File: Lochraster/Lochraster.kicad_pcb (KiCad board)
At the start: 2 copper layers, 54.6 x 53.3 mm, 25 parts, among them J1 Conn_01x04_Pin, J2 Conn_01x32_Pin, J3 Conn_01x04_Pin, J4 Conn_01x07_Pin, J5 Conn_01x08_Pin, J6 Conn_01x04_Pin, J7 Conn_01x08_Pin, J8 Conn_01x04_Pin, J9 Conn_01x04_Pin

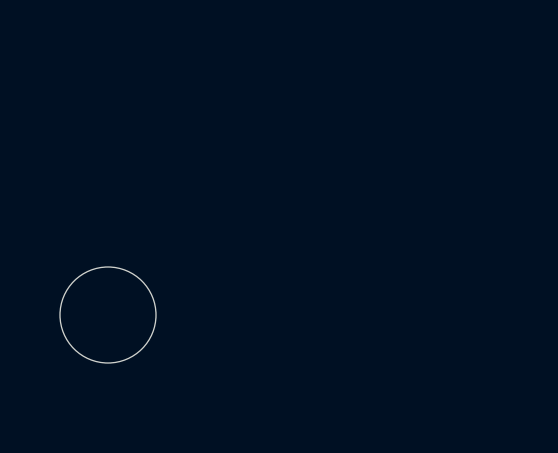
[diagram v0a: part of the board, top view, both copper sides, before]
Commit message: final version V1.0
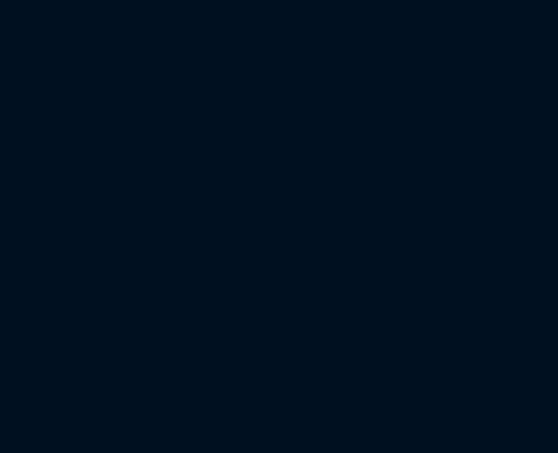
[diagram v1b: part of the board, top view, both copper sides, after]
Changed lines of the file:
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@@
     (property "ki_description" "Generic connector, single row, 01x04, script generated")
     (property "ki_keywords" "connector")
-    (attr through_hole)
+    (attr through_hole exclude_from_pos_files)
     (fp_text reference "J6" (at 0 -2.77 90) (layer "F.SilkS") hide
         (effects (font (size 1 1) (thickness 0.15)))
@@
     (property "ki_description" "Generic connector, single row, 01x08, script generated")
     (property "ki_keywords" "connector")
-    (attr through_hole)
+    (attr through_hole exclude_from_pos_files)
     (fp_text reference "J7" (at 0 -2.77 90) (layer "F.SilkS") hide
         (effects (font (size 1 1) (thickness 0.15)))
@@
     (property "ki_description" "Generic connector, single row, 01x32, script generated")
     (property "ki_keywords" "connector")
-    (attr through_hole)
+    (attr through_hole exclude_from_pos_files)
     (fp_text reference "J2" (at -1.27 -2.77 180) (layer "F.SilkS") hide
         (effects (font (size 1 1) (thickness 0.15)))
@@
     (property "ki_description" "Generic connector, single row, 01x04, script generated")
     (property "ki_keywords" "connector")
-    (attr through_hole)
+    (attr through_hole exclude_from_pos_files)
     (fp_text reference "J8" (at 0 -2.33) (layer "F.SilkS") hide
         (effects (font (size 1 1) (thickness 0.15)))
@@
     (property "ki_description" "Generic connector, single row, 01x08, script generated")
     (property "ki_keywords" "connector")
-    (attr through_hole)
+    (attr through_hole exclude_from_pos_files)
     (fp_text reference "J5" (at 0 -2.77 90) (layer "F.SilkS") hide
         (effects (font (size 1 1) (thickness 0.15)))
@@
     (property "ki_description" "Generic connector, single row, 01x07, script generated")
     (property "ki_keywords" "connector")
-    (attr through_hole)
+    (attr through_hole exclude_from_pos_files)
     (fp_text reference "J4" (at 0 -2.77 90) (layer "F.SilkS") hide
         (effects (font (size 1 1) (thickness 0.15)))
@@
     (property "ki_description" "Generic connector, single row, 01x04, script generated")
     (property "ki_keywords" "connector")
-    (attr through_hole)
+    (attr through_hole exclude_from_pos_files)
     (fp_text reference "J9" (at 0 -2.33) (layer "F.SilkS") hide
         (effects (font (size 1 1) (thickness 0.15)))
@@
     (property "ki_description" "Generic connector, single row, 01x04, script generated")
     (property "ki_keywords" "connector")
-    (attr through_hole)
+    (attr through_hole exclude_from_pos_files)
     (fp_text reference "J1" (at 0 -2.33) (layer "F.SilkS") hide
         (effects (font (size 1 1) (thickness 0.15)))
@@
     (property "ki_description" "Generic connector, single row, 01x04, script generated")
     (property "ki_keywords" "connector")
-    (attr through_hole)
+    (attr through_hole exclude_from_pos_files)
     (fp_text reference "J3" (at 0 -2.33) (layer "F.SilkS") hide
         (effects (font (size 1 1) (thickness 0.15)))
@@
         (effects (font (size 1 1) (thickness 0.15)) (justify mirror))
     )
-    (fp_line (start 0 -53.34) (end 0 0)
-      (stroke (width 0.15) (type solid)) (layer "B.SilkS"))
-    (fp_line (start 0 -53.34) (end 97.536 -53.34)
-      (stroke (width 0.15) (type solid)) (layer "B.SilkS"))
-    (fp_line (start 0 0) (end 99.06 0)
-      (stroke (width 0.15) (type solid)) (layer "B.SilkS"))
-    (fp_line (start 97.536 -53.34) (end 99.06 -51.816)
-      (stroke (width 0.15) (type solid)) (layer "B.SilkS"))
-    (fp_line (start 99.06 -40.64) (end 99.06 -51.816)
-      (stroke (width 0.15) (type solid)) (layer "B.SilkS"))
-    (fp_line (start 99.06 -1.27) (end 101.6 -3.81)
-      (stroke (width 0.15) (type solid)) (layer "B.SilkS"))
-    (fp_line (start 99.06 0) (end 99.06 -1.27)
-      (stroke (width 0.15) (type solid)) (layer "B.SilkS"))
-    (fp_line (start 101.6 -38.1) (end 99.06 -40.64)
-      (stroke (width 0.15) (type solid)) (layer "B.SilkS"))
-    (fp_line (start 101.6 -3.81) (end 101.6 -38.1)
-      (stroke (width 0.15) (type solid)) (layer "B.SilkS"))
-    (fp_circle (center 13.97 -2.54) (end 17.42 -2.54)
-      (stroke (width 0.15) (type solid)) (fill none) (layer "F.CrtYd"))
-    (fp_circle (center 15.24 -50.8) (end 18.69 -50.8)
-      (stroke (width 0.15) (type solid)) (fill none) (layer "F.CrtYd"))
     (fp_circle (center 90.17 -50.8) (end 93.62 -50.8)
       (stroke (width 0.15) (type solid)) (fill none) (layer "F.CrtYd"))
     (fp_circle (center 96.52 -2.54) (end 99.97 -2.54)
       (stroke (width 0.15) (type solid)) (fill none) (layer "F.CrtYd"))
-    (fp_line (start -6.34 -44.0036) (end 9.41 -44.0036)
-      (stroke (width 0.15) (type solid)) (layer "B.Fab"))
-    (fp_line (start -6.34 -32.1936) (end -6.34 -44.0036)
-      (stroke (width 0.15) (type solid)) (layer "B.Fab"))
-    (fp_line (start -6.34 -32.1936) (end 9.41 -32.1936)
-      (stroke (width 0.15) (type solid)) (layer "B.Fab"))
-    (fp_line (start -1.68 -12.2936) (end -1.68 -3.3026)
-      (stroke (width 0.15) (type solid)) (layer "B.Fab"))
-    (fp_line (start -1.68 -12.2936) (end 11.81 -12.2936)
-      (stroke (width 0.15) (type solid)) (layer "B.Fab"))
-    (fp_line (start -1.68 -3.3026) (end 11.81 -3.3026)
-      (stroke (width 0.15) (type solid)) (layer "B.Fab"))
-    (fp_line (start 9.41 -32.1936) (end 9.41 -44.0036)
-      (stroke (width 0.15) (type solid)) (layer "B.Fab"))
-    (fp_line (start 11.81 -12.2936) (end 11.81 -3.3026)
-      (stroke (width 0.15) (type solid)) (layer "B.Fab"))
-    (fp_rect (start 17.526 -52.07) (end 42.926 -49.53)
-      (stroke (width 0.1) (type solid)) (fill none) (layer "B.Fab"))
-    (fp_rect (start 26.67 -3.81) (end 46.99 -1.27)
-      (stroke (width 0.1) (type solid)) (fill none) (layer "B.Fab"))
     (fp_rect (start 44.45 -52.07) (end 64.77 -49.53)
       (stroke (width 0.1) (type solid)) (fill none) (layer "B.Fab"))
@@
     (fp_rect (start 92.71 -52.07) (end 97.79 -6.35)
       (stroke (width 0.1) (type solid)) (fill none) (layer "B.Fab"))
-    (fp_circle (center 13.97 -2.54) (end 17.17 -2.54)
-      (stroke (width 0.15) (type solid)) (fill none) (layer "B.Fab"))
-    (fp_circle (center 15.24 -50.8) (end 18.44 -50.8)
-      (stroke (width 0.15) (type solid)) (fill none) (layer "B.Fab"))
     (fp_circle (center 90.17 -50.8) (end 93.37 -50.8)
       (stroke (width 0.15) (type solid)) (fill none) (layer "B.Fab"))
     (fp_circle (center 96.52 -2.54) (end 99.72 -2.54)
       (stroke (width 0.15) (type solid)) (fill none) (layer "B.Fab"))
-    (fp_circle (center 13.97 -2.54) (end 17.17 -2.54)
-      (stroke (width 0.15) (type solid)) (fill none) (layer "F.Fab"))
-    (fp_circle (center 15.24 -50.8) (end 18.44 -50.8)
-      (stroke (width 0.15) (type solid)) (fill none) (layer "F.Fab"))
     (fp_circle (center 90.17 -50.8) (end 93.37 -50.8)
       (stroke (width 0.15) (type solid)) (fill none) (layer "F.Fab"))
     (fp_circle (center 96.52 -2.54) (end 99.72 -2.54)
       (stroke (width 0.15) (type solid)) (fill none) (layer "F.Fab"))
-    (pad "" np_thru_hole circle locked (at 13.97 -2.54) (size 3.2 3.2) (drill 3.2) (layers "*.Cu" "*.Mask"))
     (pad "" np_thru_hole circle locked (at 90.17 -50.8) (size 3.2 3.2) (drill 3.2) (layers "*.Cu" "*.Mask"))
     (pad "" np_thru_hole circle locked (at 96.52 -2.54) (size 3.2 3.2) (drill 3.2) (layers "*.Cu" "*.Mask"))
@@
     (effects (font (size 0.5 0.5) (thickness 0.1) bold) (justify left bottom))
   )
+  (dimension (type aligned) (layer "F.Fab")
+    (pts (xy 211.013 105.26) (xy 211.013 51.92))
+    (height 11.43)
+    (gr_text "53,3400 mm" (at 221.293 78.59 90) (layer "F.Fab")
+      (effects (font (size 1 1) (thickness 0.15)))
+    )
+    (format (prefix "") (suffix "") (units 3) (units_format 1) (precision 4))
+    (style (thickness 0.1) (arrow_length 1.27) (text_position_mode 0) (extension_height 0.58642) (extension_offset 0.5) keep_text_aligned)
+  )
+  (dimension (type aligned) (layer "F.Fab")
+    (pts (xy 156.403 51.92) (xy 211.013 51.92))
+    (height -3.81)
+    (gr_text "54,6100 mm" (at 183.708 46.96) (layer "F.Fab")
+      (effects (font (size 1 1) (thickness 0.15)))
+    )
+    (format (prefix "") (suffix "") (units 3) (units_format 1) (precision 4))
+    (style (thickness 0.1) (arrow_length 1.27) (text_position_mode 0) (extension_height 0.58642) (extension_offset 0.5) keep_text_aligned)
+  )
   (segment (start 162.753 64.65) (end 160.243 64.65) (width 1) (layer "F.Cu") (net 1))
